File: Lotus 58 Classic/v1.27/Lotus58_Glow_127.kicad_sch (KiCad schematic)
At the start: 127 parts, among them J1 PJ-320A, J2 Conn_01x02, P1 OLED, SW1 Kailh hotswap MX socket, SW10 Kailh hotswap MX socket, SW11 Kailh hotswap MX socket, SW12 Kailh hotswap MX socket, SW13 Kailh hotswap MX socket, SW14 Kailh hotswap MX socket, SW15 Kailh hotswap MX socket, SW16 Kailh hotswap MX socket, SW17 Kailh hotswap MX socket, SW18 Kailh hotswap MX socket, SW19 Kailh hotswap MX socket, SW2 Kailh hotswap MX socket, SW20 Kailh hotswap MX socket, SW21 Kailh hotswap MX socket, SW22 Kailh hotswap MX socket, SW23 Kailh hotswap MX socket, SW24 Kailh hotswap MX socket, SW25 Kailh hotswap MX socket, SW26 Kailh hotswap MX socket, SW27 Kailh hotswap MX socket, SW28 Kailh hotswap MX socket, SW29 Kailh hotswap MX socket, SW3 Kailh hotswap MX socket, SW30 Rotary_Encoder_Switch, SW31 Rotary_Encoder_Switch, SW4 Kailh hotswap MX socket, SW5 Kailh hotswap MX socket, SW6 Kailh hotswap MX socket, SW7 Kailh hotswap MX socket, SW8 Kailh hotswap MX socket, SW9 Kailh hotswap MX socket, U1 ProMicro, U2 SRV05-4

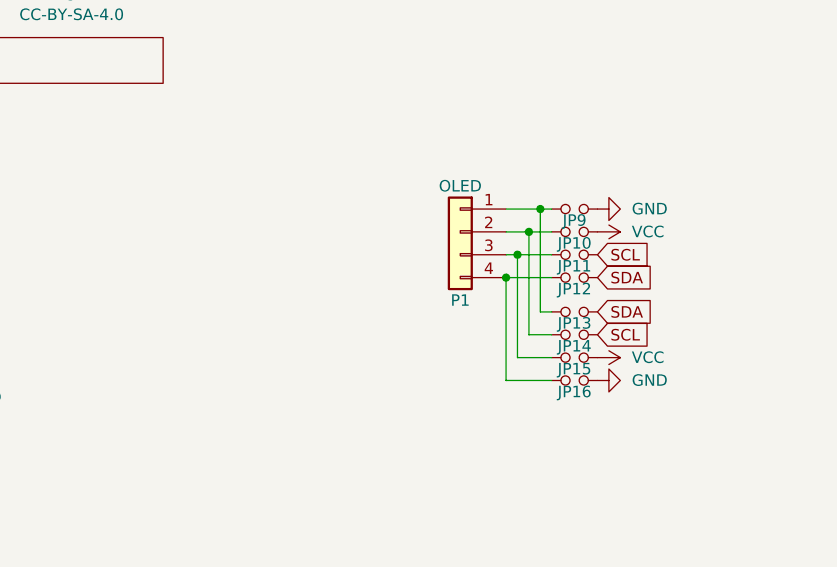
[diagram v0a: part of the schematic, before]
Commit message: Created STEP files for 3D model
Signed-off-by: TweetyDaBird <markus.knutsson@tweety.se>
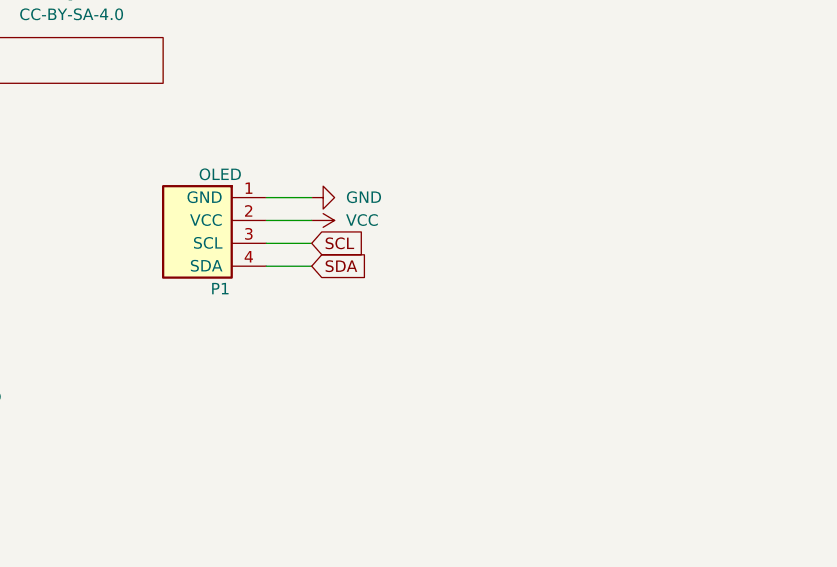
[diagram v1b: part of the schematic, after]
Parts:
- removed JP10, JP11, JP12, JP13, JP14, JP15, JP16, JP9: Jumper_NO_Small, Keyboard Common:Jumper_min_v2, symbol Device:Jumper_NO_Small
- removed P1: OLED, KiCad-SSD1306-0.91-OLED-4pin-128x32:SSD1306-0.91-OLED-4pin-128x32, symbol Connector_Generic:Conn_01x04
- added P1: OLED, Keyboard Common:SSD1306-0.91-OLED-4pin-128x32 doublesided, symbol Keyboard Common:OLED_4pin
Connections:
- net GND: now also P1.1 (GND)
- net SCL: now also P1.3 (SCL)
- net SDA: now also P1.4 (SDA)
- net VCC: now also P1.2 (VCC)
- new net: P1.A (0), P1.B (0), P1.C (0), P1.D (0)
